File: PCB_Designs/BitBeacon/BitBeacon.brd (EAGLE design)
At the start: 30.5 x 33 mm, 100 parts, among them IC1 AD8603UJ, IC2 AD8603UJ, IC3 AD8603UJ, IC4 AD8603UJ

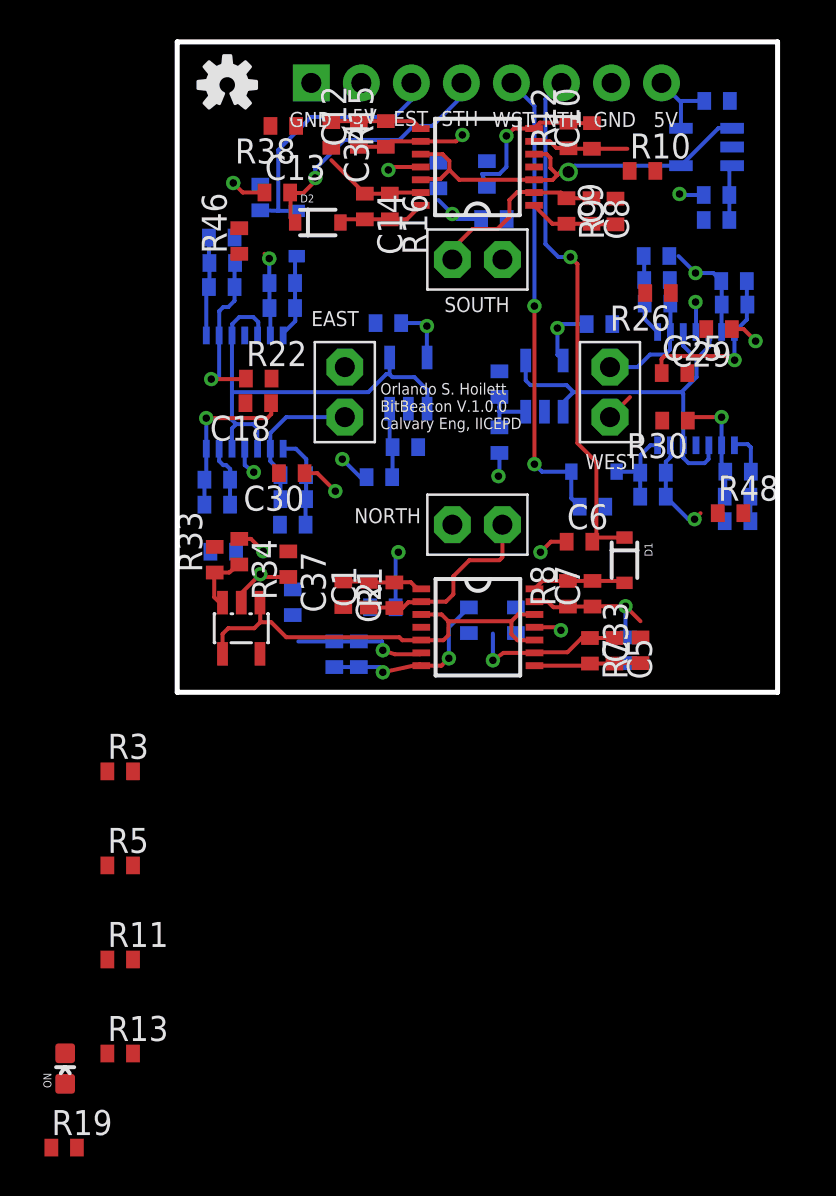
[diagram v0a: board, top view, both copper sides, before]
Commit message: made minor changes to BitBeacon
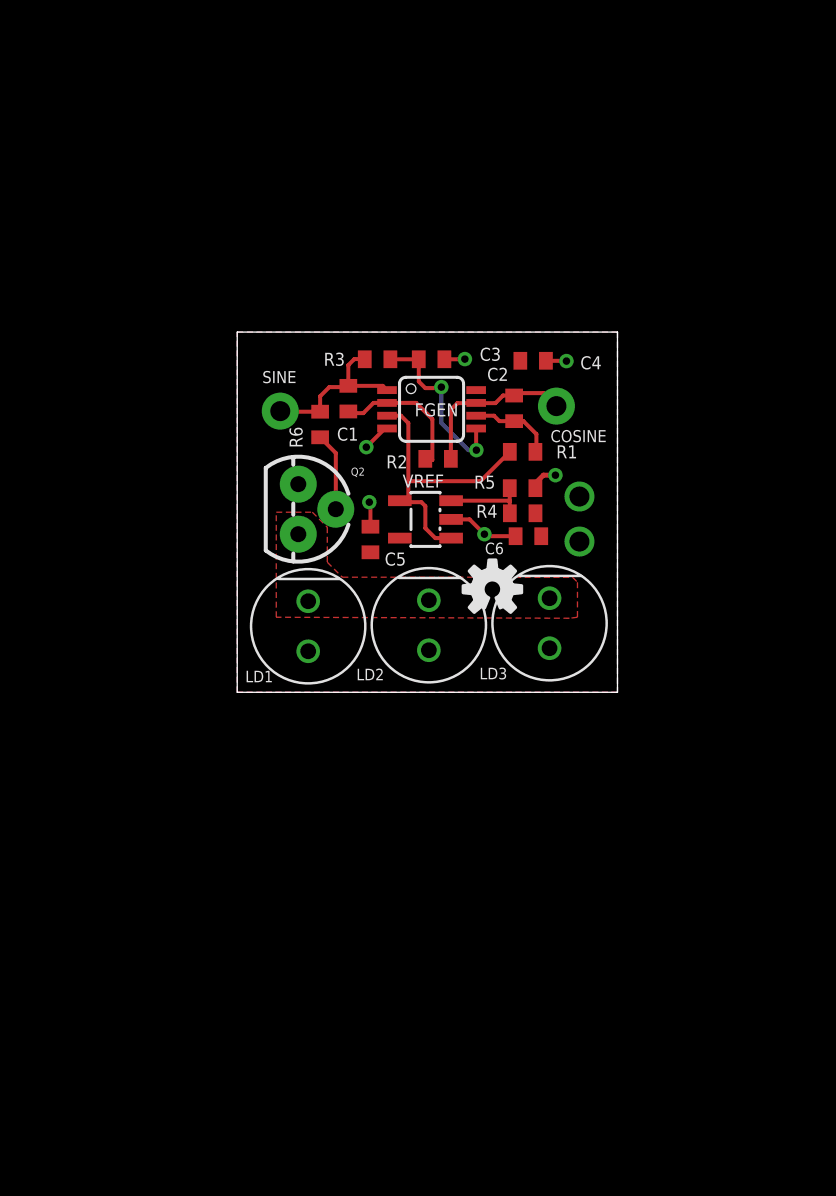
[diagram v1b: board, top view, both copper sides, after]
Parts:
- removed C10, C12, C14, C15, C17, C19, C21, C22, C24, C26, C28, C7, C8: 22p, resistor:C0402
- removed C11, C16, C18, C23, C25, C33, C34, C35, C36, C9: (no value), resistor:C0402
- removed C13, C20, C27, C29, C30, C31, C32, C37, C38, C39, C40: 100n, resistor:C0402
- removed D1, D2, D3, D4: 250mA/100V, SparkFun-DiscreteSemi:SOD-323
- removed E-AMP, S-AMP, W-AMP: AD8609RU, analog-devices:TSSOP14
- removed E-PD1, N-PD1, S-PD1, W-PD1: BPW46, Orlando:PIN-PHOTODIODE
- removed IC1, IC2, IC3, IC4: AD8603UJ, analog-devices:SOT23-5
- removed N-AMP: AD8608, analog-devices:TSSOP14
- removed ON: GREEN, SparkFun-LED:LED-0603
- removed R10, R14, R18, R19, R22, R26, R30, R33, R34, R36, R38, R39, R40, R41, R42, R43, R44, R46, R48: (no value), resistor:R0402
- removed R11, R12, R13, R15, R16, R20, R23, R24, R28, R31, R32, R7, R8: 1M, resistor:R0402
- removed R17, R25, R9: 1k, resistor:R0402
- added BATTERY: BATT-CONNECT, OrlandoRonMod:HOLE
- added FGEN: (no value), analog-devices:MSOP08
- added JP1: M01NOSILK-KIT, SparkFun-Connectors:1X01NS-KIT
- added LED1, LED2, LED3: LED, Orlando:LED
- added Q2: (no value), SparkFun-DiscreteSemi:TO-92
- added VREF: (no value), analog-devices:SOT23-5
- C1, C3: value 22p -> 1n
- C2: value (none) -> 1n
- C4: value (none) -> 100n
- C5: value 22p -> 100n
- JP2: value (none) -> M01NOSILK-KIT; device SparkFun-Connectors:1X08_PIN1_NO_SILK -> SparkFun-Connectors:1X01NS-KIT
- R1: value 1k -> 22k
- R2: value (none) -> 22k
- R3, R4, R5: value 1M -> 22k
- R6: value (none) -> 10k-50k
- moved LOGO1 28.9 mm to (16.0, 5.23)
- moved R5 28.0 mm to (17.5, 10.4)
- moved R3 24.7 mm to (10.2, 16.9), turned to 180 degrees
- moved JP2 20.6 mm to (19.3, 14.5)
- moved C3 15.8 mm to (12.9, 16.9), flipped to the top, turned to 180 degrees
- moved R6 14.1 mm to (7.25, 13.6), flipped to the top
- moved C5 13.6 mm to (9.81, 7.76), turned to 90 degrees
- moved C4 13.6 mm to (18.1, 16.8), flipped to the top, turned to 180 degrees
- moved C2 12.8 mm to (17.1, 14.4)
- moved R4 11.0 mm to (17.5, 9.09), flipped to the top, turned to 0 degrees
- moved R2 10.4 mm to (13.2, 11.9), flipped to the top, turned to 180 degrees
- moved C1 10.0 mm to (8.69, 14.9)
- moved R1 9.77 mm to (17.5, 12.2), turned to 0 degrees
- moved C6 2.61 mm to (17.8, 7.92), turned to 180 degrees
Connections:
- removed net 1/2-VDD-E: E-AMP.10, E-AMP.12, E-AMP.3, E-AMP.5, IC3.1, IC3.4
- removed net 1/2-VDD-N: IC1.1, IC1.4, N-AMP.10, N-AMP.12, N-AMP.3, N-AMP.5
- removed net 1/2-VDD-S: IC2.1, IC2.4, S-AMP.10, S-AMP.12, S-AMP.3, S-AMP.5
- removed net 1/2-VDD-W: IC4.1, IC4.4, W-AMP.10, W-AMP.12, W-AMP.3, W-AMP.5
- removed net E-OUT: C20.2, D3.C, JP2.3, R11.2
- removed net N$1: C1.1, N-AMP.2, N-PD1.2, R1.1
- removed net N$10: C7.1, N-AMP.13, R36.1, R8.1
- removed net N$11: C7.2, D1.A, N-AMP.14, R8.2
- removed net N$12: C10.1, R10.1, R12.1, S-AMP.6
- removed net N$13: C10.2, C11.1, R12.2, S-AMP.7
- removed net N$14: C12.1, R14.1, R15.1, S-AMP.9
- removed net N$15: C12.2, C34.1, R15.2, S-AMP.8
- removed net N$16: IC2.3, R39.1, R40.2
- removed net N$17: IC3.3, R41.1, R42.2
- removed net N$18: IC4.3, R43.1, R44.2
- removed net N$19: C15.1, E-AMP.2, E-PD1.2, R17.1
- removed net N$20: C15.2, C16.1, E-AMP.1, R17.2
- removed net N$21: C17.1, E-AMP.6, R18.1, R20.1
- removed net N$22: C17.2, C18.1, E-AMP.7, R20.2
- removed net N$23: C19.1, E-AMP.9, R22.1, R23.1
- removed net N$24: C19.2, C35.1, E-AMP.8, R23.2
- removed net N$25: C28.1, R32.1, R48.1, W-AMP.13
- removed net N$26: C21.1, E-AMP.13, R24.1, R46.1
- removed net N$27: C2.2, R2.2
- removed net N$28: C22.1, R25.1, W-AMP.2, W-PD1.2
- removed net N$29: C22.2, C23.1, R25.2, W-AMP.1
- removed net N$30: C24.1, R26.1, R28.1, W-AMP.6
- removed net N$31: C24.2, C25.1, R28.2, W-AMP.7
- removed net N$32: C26.1, R30.1, R31.1, W-AMP.9
- removed net N$33: C26.2, C36.1, R31.2, W-AMP.8
- removed net N$34: C4.2, R6.2
- removed net N$35: C33.2, R36.2
- removed net N$36: C34.2, R38.2
- removed net N$37: C11.2, R14.2
- removed net N$38: C9.2, R10.2
- removed net N$39: C35.2, R46.2
- removed net N$4: C8.1, R9.1, S-AMP.2, S-PD1.2
- removed net N$40: C18.2, R22.2
- removed net N$41: C16.2, R18.2
- removed net N$42: C36.2, R48.2
- removed net N$43: C25.2, R30.2
- removed net N$44: C14.2, D2.A, R16.2, S-AMP.14
- removed net N$45: C23.2, R26.2
- removed net N$46: C21.2, D3.A, E-AMP.14, R24.2
- removed net N$47: C28.2, D4.A, R32.2, W-AMP.14
- removed net N$48: ON.C, R19.2
- removed net N-OUT: C6.2, D1.C, JP2.6, R3.2
- removed net S-AMP: C8.2, C9.1, R9.2, S-AMP.1
- removed net S-OUT: C13.2, D2.C, JP2.4, R5.2
- removed net W-OUT: C27.2, D4.C, JP2.5, R13.2
- new net COSINE: C2.1, FGEN.7, JP2.1, R2.1
- new net SINE: C1.2, FGEN.1, JP1.1, R3.2, R6.2
- net 5V: now also BATTERY.P$2, C4.2, C5.1, C6.1, FGEN.8, LED1.A, LED2.A, LED3.A, R4.2, VREF.5; no longer C29.2, C30.2, C31.2, C32.2, C37.1, C38.1, C39.1, C40.1, E-AMP.4, IC1.5, IC2.5, IC3.5, IC4.5, JP2.2, JP2.8, N-AMP.4, ON.A, R33.2, R39.2, R41.2, R43.2, S-AMP.4, W-AMP.4
- net GND: now also BATTERY.P$1, C3.1, C4.1, C5.2, C6.2, FGEN.4, Q2.1, R5.2, VREF.2; no longer C13.1, C20.1, C27.1, C29.1, C30.1, C31.1, C32.1, C37.2, C38.2, C39.2, C40.2, C6.1, E-AMP.11, E-PD1.1, IC1.2, IC2.2, IC3.2, IC4.2, JP2.1, JP2.7, N-AMP.11, N-PD1.1, R11.1, R13.1, R19.1, R3.1, R34.1, R40.1, R42.1, R44.1, R5.1, S-AMP.11, S-PD1.1, W-AMP.11, W-PD1.1
- net N$2: now also C3.2, FGEN.5, R3.1; no longer C14.1, R16.1, R38.1, S-AMP.13
- net N$3: now also C1.1, FGEN.2, R2.2; no longer C1.2, C2.1, N-AMP.1, R1.2
- net N$5: now also C2.2, FGEN.6, R1.2; no longer C3.1, N-AMP.6, R2.1, R4.1
- net N$6: now also FGEN.3, R1.1, VREF.1, VREF.4; no longer C3.2, C4.1, N-AMP.7, R4.2
- net N$7: now also R4.1, R5.1, VREF.3; no longer C5.1, N-AMP.9, R6.1, R7.1
- net N$8: now also LED1.C, LED2.C, LED3.C, Q2.3; no longer C33.1, C5.2, N-AMP.8, R7.2
- net N$9: now also Q2.2, R6.1; no longer IC1.3, R33.1, R34.2
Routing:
- net N-OUT: track 26.6 -> 0.00 mm, vias 1 -> 0
- net W-OUT: track 23.8 -> 0.00 mm, vias 2 -> 0
- net 1/2-VDD-E: track 23.5 -> 0.00 mm
- net 1/2-VDD-N: track 23.2 -> 0.00 mm
- net 5V: track 22.7 -> 0.00 mm, vias 9 -> 0
- net 1/2-VDD-S: track 21.3 -> 0.00 mm, vias 1 -> 0
- net 1/2-VDD-W: track 21.3 -> 0.00 mm
- net E-OUT: track 13.6 -> 0.00 mm
- net S-OUT: track 13.4 -> 0.00 mm, vias 1 -> 0
- net N$1: track 10.0 -> 0.00 mm
- net N$4: track 9.43 -> 0.00 mm
- net N$31: track 8.88 -> 0.00 mm, vias 1 -> 0
- net SINE: track 0.00 -> 8.54 mm
- net N$23: track 8.51 -> 0.00 mm, vias 1 -> 0
- net COSINE: track 0.00 -> 8.49 mm
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- added copper zone on layer 1, net N$8
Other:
- board size 30.5 x 33 mm -> 19.3 x 18.3 mm
- board text added: "Battery"
- board text added: "COSINE"
- board text added: "LD1"
- board text added: "LD2"
- board text added: "LD3"
- board text added: "Orlando S. Hoilett BIT Beacon Sig V.1.0 Calvary Eng, IICEPD"
- board text added: "SINE"
- board text removed: "5V"
- board text removed: "EAST"
- board text removed: "EST"
- board text removed: "GND"
- board text removed: "NORTH"
- board text removed: "NTH"
- board text removed: "Orlando S. Hoilett BitBeacon V.1.0.0 Calvary Eng, IICEPD"
- board text removed: "SOUTH"
- board text removed: "STH"
- board text removed: "WEST"
- board text removed: "WST"
